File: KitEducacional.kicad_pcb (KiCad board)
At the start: 2 copper layers, 110 x 86 mm, 45 parts, among them J1 Serial 1, J10 D4, J11 D5, J12 D6, J13 D7, J14 D8, J15 D9, J16 D10, J17 D11, J18 D12, J19 D13, J2 Serial 2, J20 D14, J21 D15, J22 A0, J23 A1, J24 A2, J25 A3, J26 A4, J27 A5, J28 A6, J29 A7, J3 Serial 3, J4 I²C, J5 SPI, J6 D0, J7 D1, J8 D2, J9 D3, SW1 SW_Push, SW2 SW_Push, SW3 SW_Push, SW4 SW_Push, SW5 SW_Push, U1 ESP32-WROOM-32

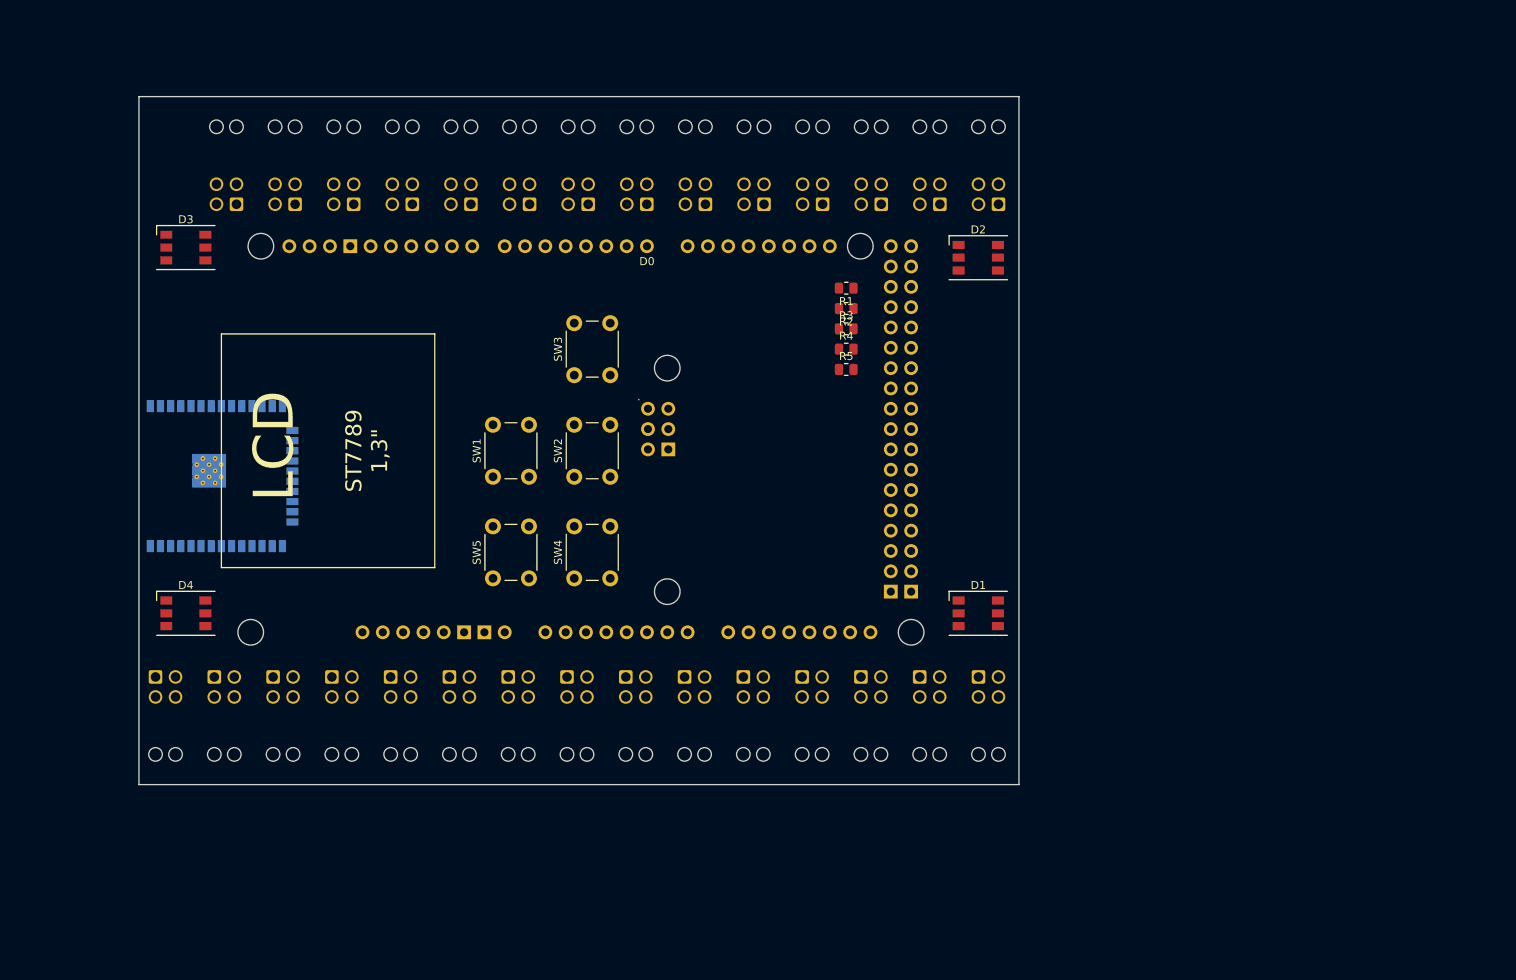
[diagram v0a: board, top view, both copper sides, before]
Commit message: goto mini-fit
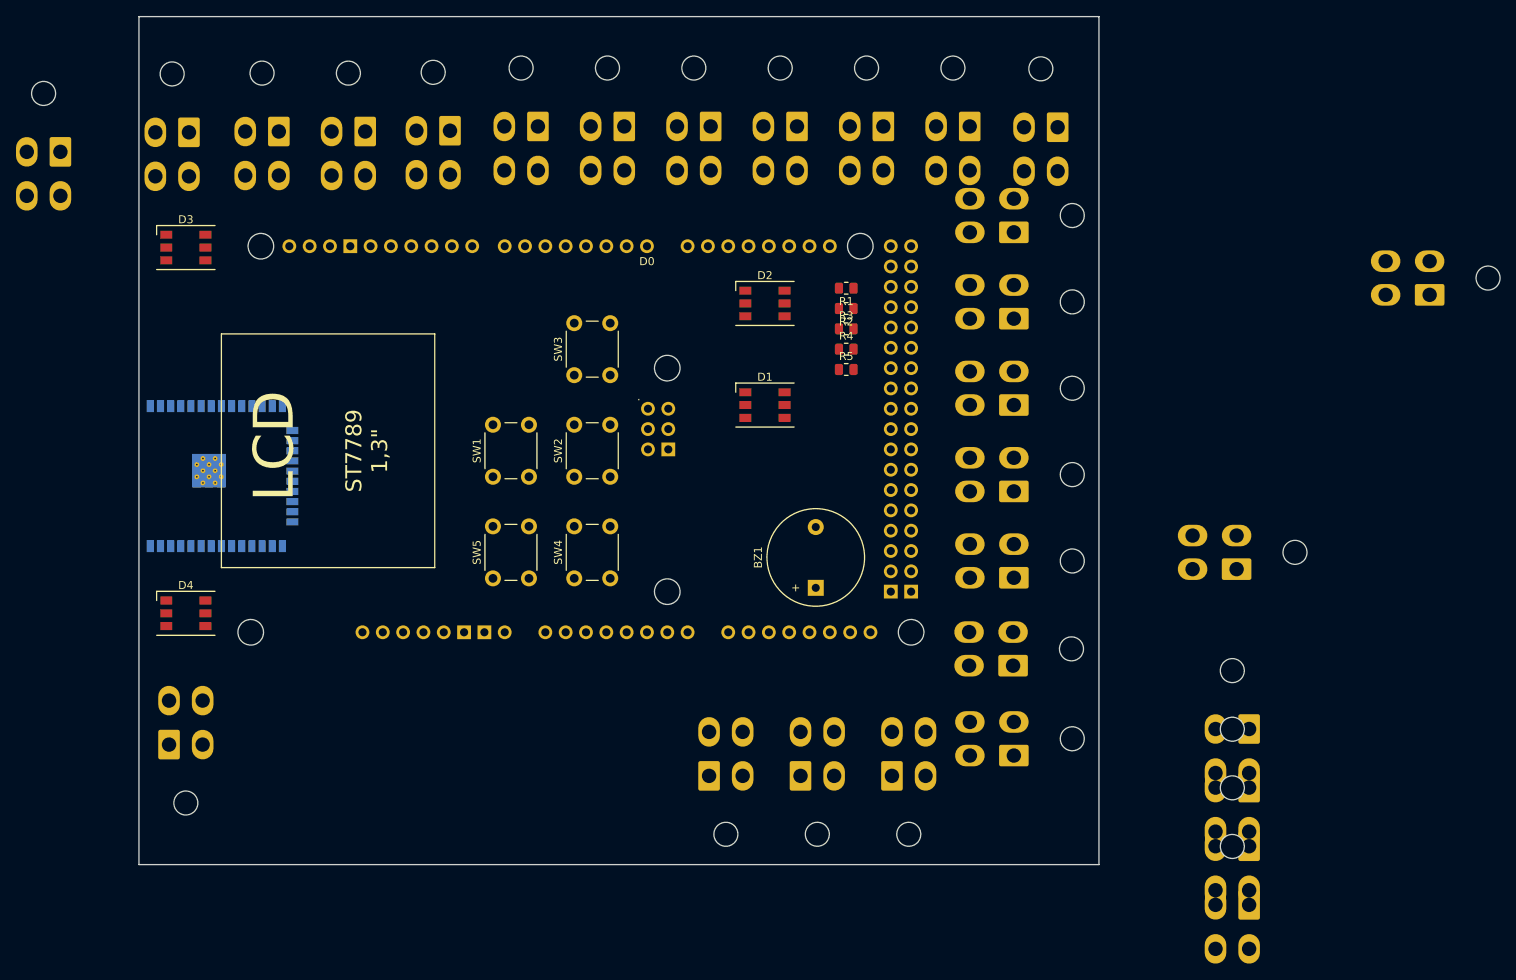
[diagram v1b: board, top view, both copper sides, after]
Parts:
- added BZ1: Buzzer, Buzzer_Beeper:Buzzer_12x9.5RM7.6, F.Cu at (186.7, 108.6)
- J1, J10, J11, J12, J13, J14, J15, J16, J17, J18, J19, J2, J20, J21, J22, J23, J24, J25, J26, J27, J28, J29, J3, J4, J5, J6, J7, J8, J9: footprint Connector_Molex:Molex_Nano-Fit_105314-xx04_2x02_P2.50mm_Horizontal -> Connector_Molex:Molex_Mini-Fit_Jr_5569-04A2_2x02_P4.20mm_Horizontal
- moved J13 152.3 mm to (263.4, 72.0), turned to 90 degrees
- moved J27 148.0 mm to (240.9, 148.2), turned to 180 degrees
- moved J26 137.7 mm to (240.9, 140.9), turned to 180 degrees
- moved J25 127.5 mm to (240.9, 133.5), turned to 180 degrees
- moved J24 117.3 mm to (240.9, 126.2), turned to 180 degrees
- moved J14 114.4 mm to (211.5, 64.1), turned to 90 degrees
- moved J4 102.5 mm to (108.3, 51.6), turned to 180 degrees
- moved J23 99.5 mm to (239.3, 106.2)
- moved J8 77.1 mm to (119.6, 51.5), turned to 180 degrees
- moved J7 75.6 mm to (130.4, 51.5), turned to 180 degrees
- moved J21 74.0 mm to (184.8, 132.1), turned to 0 degrees
- moved J22 73.0 mm to (173.4, 132.1), turned to 0 degrees
- moved J10 72.2 mm to (162.8, 50.9), turned to 180 degrees
- moved J12 71.1 mm to (196.2, 132.1), turned to 0 degrees
- moved J20 69.3 mm to (211.4, 118.3)
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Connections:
- A1 pad D23: unconnected-(A1-PadD23) -> D23
- A1 pad D25: unconnected-(A1-PadD25) -> D25
- A1 pad D27: unconnected-(A1-PadD27) -> D27
- A1 pad D29: unconnected-(A1-PadD29) -> D29
- A1 pad D31: unconnected-(A1-PadD31) -> D31
- A1 pad D33: unconnected-(A1-PadD33) -> D33
- A1 pad D34: unconnected-(A1-PadD34) -> D34
- A1 pad D35: unconnected-(A1-PadD35) -> D35
- A1 pad D36: unconnected-(A1-PadD36) -> D36
- A1 pad D37: unconnected-(A1-PadD37) -> D37
- A1 pad D38: unconnected-(A1-PadD38) -> D38
- A1 pad D39: unconnected-(A1-PadD39) -> D39
- A1 pad D40: unconnected-(A1-PadD40) -> D40
- A1 pad D41: unconnected-(A1-PadD41) -> D41
- A1 pad D44: unconnected-(A1-PadD44) -> D44
- A1 pad D45: unconnected-(A1-PadD45) -> D45
- A1 pad D46: unconnected-(A1-PadD46) -> D46
- A1 pad D47: unconnected-(A1-PadD47) -> D47
- J13 pad 1: unconnected-(J13-Pin_1-Pad1) -> D23
- J13 pad 2: unconnected-(J13-Pin_2-Pad2) -> D25
- J14 pad 1: unconnected-(J14-Pin_1-Pad1) -> D27
- J14 pad 2: unconnected-(J14-Pin_2-Pad2) -> D29
- J15 pad 1: unconnected-(J15-Pin_1-Pad1) -> D31
- J15 pad 2: unconnected-(J15-Pin_2-Pad2) -> D33
- J16 pad 1: unconnected-(J16-Pin_1-Pad1) -> D35
- J16 pad 2: unconnected-(J16-Pin_2-Pad2) -> D37
- J17 pad 1: unconnected-(J17-Pin_1-Pad1) -> D39
- J17 pad 2: unconnected-(J17-Pin_2-Pad2) -> D41
- J18 pad 1: unconnected-(J18-Pin_1-Pad1) -> D34
- J18 pad 2: unconnected-(J18-Pin_2-Pad2) -> D36
- J19 pad 1: unconnected-(J19-Pin_1-Pad1) -> D38
- J19 pad 2: unconnected-(J19-Pin_2-Pad2) -> D40
- J20 pad 1: unconnected-(J20-Pin_1-Pad1) -> D45
- J20 pad 2: unconnected-(J20-Pin_2-Pad2) -> D47
- J21 pad 1: unconnected-(J21-Pin_1-Pad1) -> D44
- J21 pad 2: unconnected-(J21-Pin_2-Pad2) -> D46
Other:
- board size 110 x 86 mm -> 120 x 106 mm
